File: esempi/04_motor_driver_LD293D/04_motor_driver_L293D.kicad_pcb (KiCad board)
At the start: 2 copper layers, 38.1 x 38.1 mm, 24 parts, among them IC1 L293D, P1 MOTOR1_DIRECTION, P2 MOTOR1_ENABLE, P3 CONN_01X02, P4 MOTOR2_ENABLE, P5 CONN_01X02, P6 MOTOR2_DIRECTION, P7 CONN_01X01, P8 CONN_01X01, P9 CONN_01X01, Q1 Q_NPN_BCE, Q2 Q_NPN_BCE

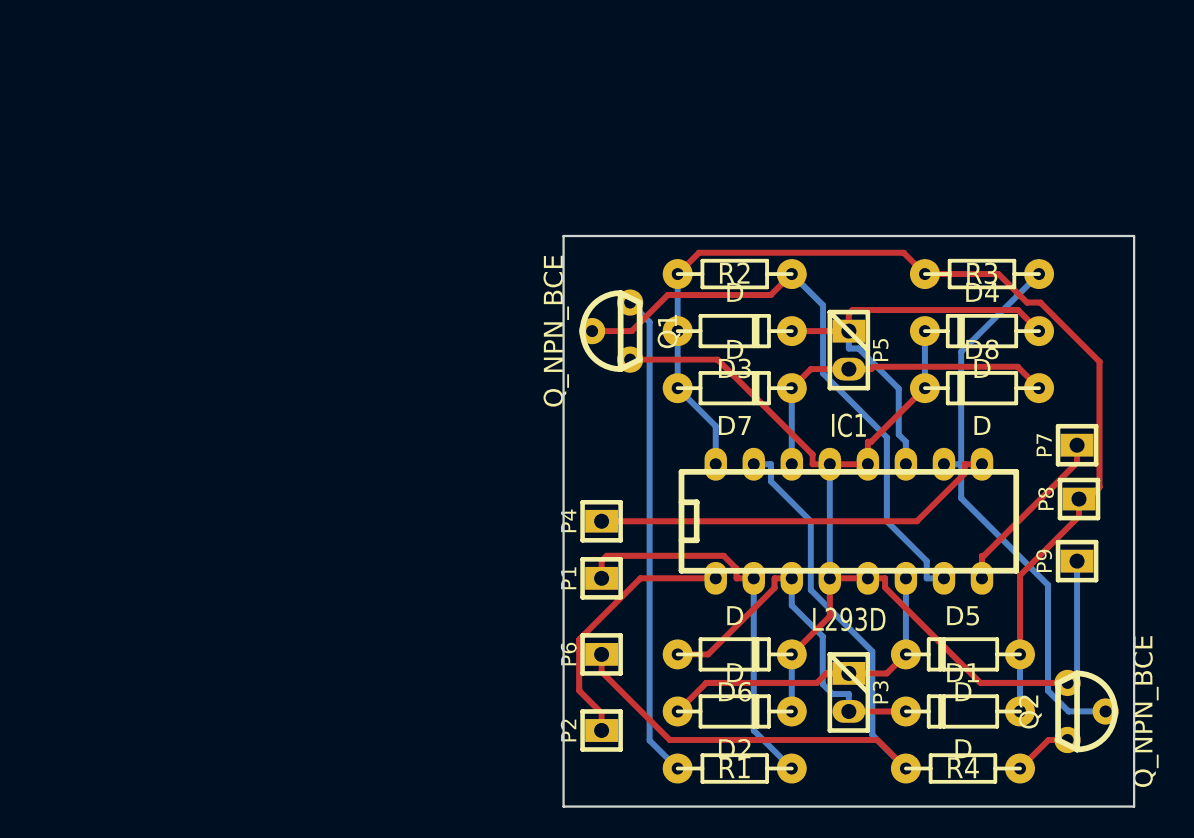
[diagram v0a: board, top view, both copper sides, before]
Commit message: Modifiche alla board per uso su motori recuperati da macchinetta caffe
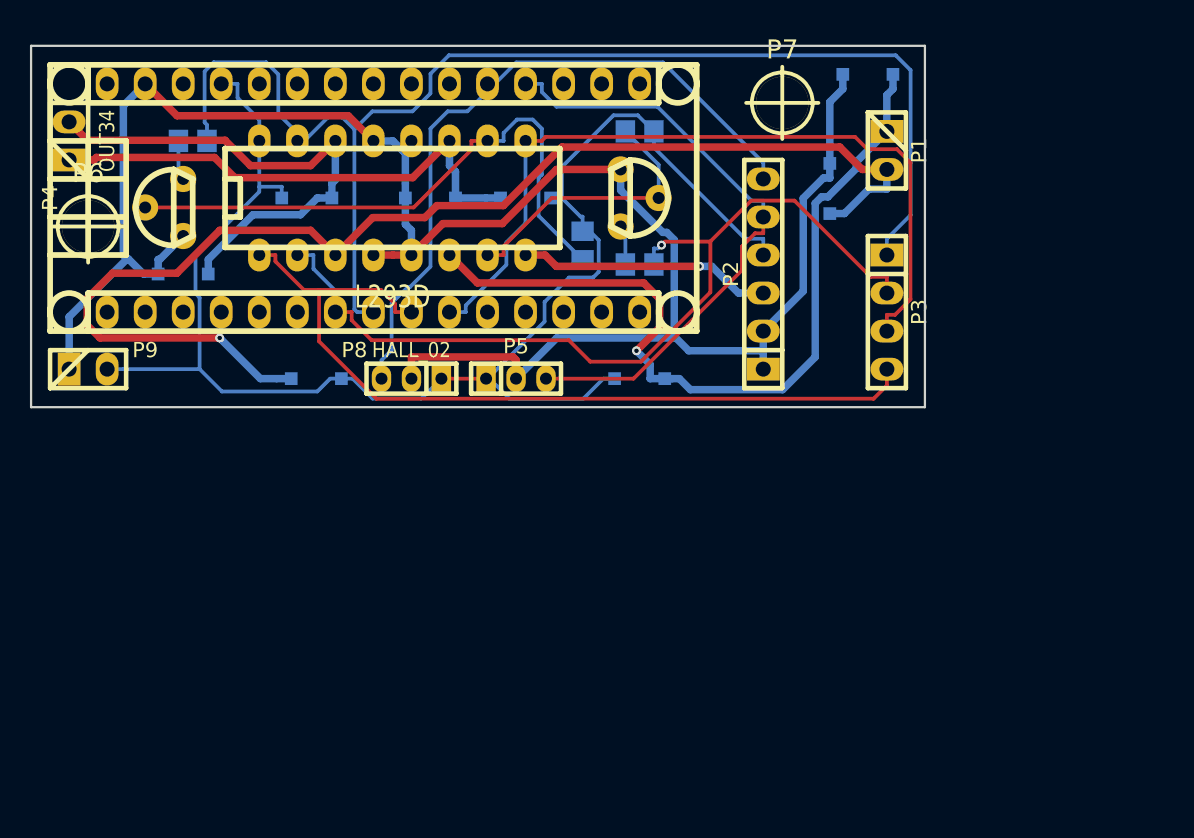
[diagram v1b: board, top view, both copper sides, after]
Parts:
- added J1: Arduino_Nano_Header, w_conn_misc:arduino_nano_header, F.Cu at (114.3, 73.7)
- D1, D2, D3, D4, D5, D6, D7, D8: footprint w_pth_diodes:diode_do35 -> w_smd_diode:sod123; moved to B.Cu
- P1: value MOTOR1_DIRECTION -> OUT12; footprint w_pin_strip:pin_strip_1 -> w_pin_strip:pin_strip_2
- P2: value MOTOR1_ENABLE -> ALIM_HALL; footprint w_pin_strip:pin_strip_1 -> w_pin_strip:pin_strip_6
- P3: value CONN_01X02 -> MOTOR_CTR; footprint w_pin_strip:pin_strip_2 -> w_pin_strip:pin_strip_4
- P4: value MOTOR2_ENABLE -> OUT34; footprint w_pin_strip:pin_strip_1 -> w_pin_strip:pin_strip_2
- P5: value CONN_01X02 -> HALL_01; footprint w_pin_strip:pin_strip_2 -> w_pin_strip:pin_strip_2mm_3
- P6: value MOTOR2_DIRECTION -> HOLE1; footprint w_pin_strip:pin_strip_1 -> w_details:hole_3mm5
- P7: value CONN_01X01 -> HOLE2; footprint w_pin_strip:pin_strip_1 -> w_details:hole_3mm5
- P8: value CONN_01X01 -> HALL_02; footprint w_pin_strip:pin_strip_1 -> w_pin_strip:pin_strip_2mm_3
- P9: value CONN_01X01 -> ING5V; footprint w_pin_strip:pin_strip_1 -> w_pin_strip:pin_strip_2
- R1, R2, R3, R4: footprint w_pth_resistors:RC03 -> w_smd_resistors:r_0805; moved to B.Cu
- moved Q2 69.1 mm to (101.0, 74.3), turned to 90 degrees
- moved P9 67.3 mm to (95.2, 85.1), turned to 0 degrees
- moved R4 66.3 mm to (102.2, 69.8)
- moved D5 53.4 mm to (109.9, 73.7), turned to 0 degrees
- moved P8 45.3 mm to (116.8, 85.7), turned to 180 degrees
- moved D6 44.7 mm to (101.6, 78.7), turned to 180 degrees
- moved P6 44.6 mm to (95.2, 75.6), turned to 0 degrees
- moved P4 43.7 mm to (94.0, 69.8)
- moved D2 43.5 mm to (147.3, 65.4), turned to 180 degrees
- moved D8 39.0 mm to (118.1, 73.7)
- moved IC1 37.4 mm to (115.6, 73.7)
- moved P1 34.3 mm to (148.6, 70.5), turned to 270 degrees
- moved R1 34.2 mm to (132.1, 78.1), turned to 0 degrees
- moved P2 32.3 mm to (140.3, 78.7)
- moved D1 31.0 mm to (132.1, 85.7), turned to 0 degrees
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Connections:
- D2 pad 1: Net-(D2-Pad1) -> Net-(D1-Pad2)
- D5 pad 2: Net-(D2-Pad1) -> Net-(D5-Pad2)
- D6 pad 1: Net-(D1-Pad2) -> Net-(D5-Pad2)
- IC1 pad 1: Net-(IC1-Pad1) -> 1,2EN
- IC1 pad 11: Net-(D3-Pad2) -> Net-(D7-Pad2)
- IC1 pad 14: Net-(D7-Pad2) -> Net-(D5-Pad2)
- IC1 pad 15: Net-(IC1-Pad15) -> 3,4DIR
- IC1 pad 2: Net-(IC1-Pad2) -> 1,2DIR
- IC1 pad 3: Net-(D1-Pad2) -> Net-(D3-Pad2)
- IC1 pad 6: Net-(D2-Pad1) -> Net-(D1-Pad2)
- IC1 pad 9: Net-(IC1-Pad9) -> 3,4EN
- P1 pad 1: Net-(IC1-Pad2) -> Net-(D1-Pad2)
- P2 pad 1: Net-(IC1-Pad1) -> GND
- P3 pad 1: Net-(D2-Pad1) -> 3,4DIR
- P3 pad 2: Net-(D1-Pad2) -> 1,2DIR
- P4 pad 1: Net-(IC1-Pad9) -> Net-(D7-Pad2)
- P5 pad 1: Net-(D3-Pad2) -> +5V
- P5 pad 2: Net-(D7-Pad2) -> GND
- P6 pad 1: Net-(IC1-Pad15) -> (no net)
- P7 pad 1: VCC -> (no net)
- R1 pad 1: Net-(IC1-Pad2) -> 1,2DIR
- R4 pad 1: Net-(IC1-Pad15) -> 3,4DIR
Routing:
- net 3,4DIR: track 0.00 -> 87.0 mm
- net GND: track 74.8 -> 135.9 mm
- net 1,2DIR: track 0.00 -> 58.7 mm, vias 0 -> 1
- net 1,2EN: track 0.00 -> 56.7 mm
- net Net-(D3-Pad2): track 29.2 -> 82.3 mm, vias 0 -> 1
- net 3,4EN: track 0.00 -> 52.9 mm
- net Net-(IC1-Pad15): track 49.4 -> 0.00 mm
- net Net-(J1-Pad20): track 0.00 -> 46.5 mm
- net Net-(J1-Pad19): track 0.00 -> 41.1 mm
- net Net-(D5-Pad2): track 0.00 -> 34.5 mm
- net +5V: track 71.7 -> 102.4 mm
- net Net-(D1-Pad2): track 25.0 -> 55.1 mm, vias 0 -> 1
- net Net-(Q1-Pad1): track 32.4 -> 2.67 mm
- net Net-(IC1-Pad9): track 27.3 -> 0.00 mm
- net Net-(IC1-Pad2): track 26.2 -> 0.00 mm
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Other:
- board size 38.1 x 38.1 mm -> 59.7 x 24.1 mm
- net class Default: trace_width 0.4 -> 0.25; via_dia 1.2 -> 0.6; via_drill 0.8 -> 0.4
- net class Motor added: clearance 0.3, trace_width 0.5, via_dia 0.6, via_drill 0.4
